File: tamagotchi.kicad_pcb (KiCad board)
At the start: 2 copper layers, 48 x 87 mm, 9 parts, among them SW1 SW_Push, SW2 SW_Push, SW3 SW_Push, U1 XIAO-ESP32-C3-SMD, U2 HS96L03W2C03

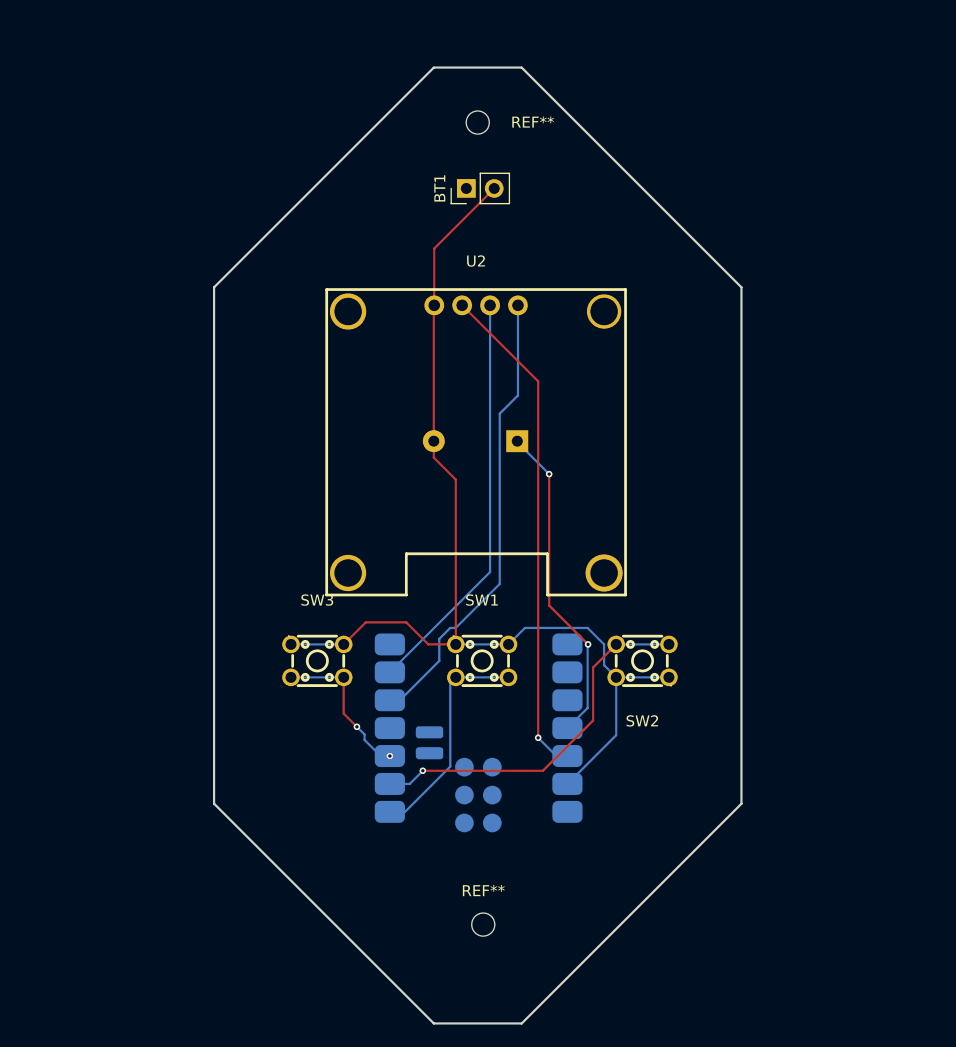
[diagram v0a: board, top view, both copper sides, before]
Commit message: Add files via upload
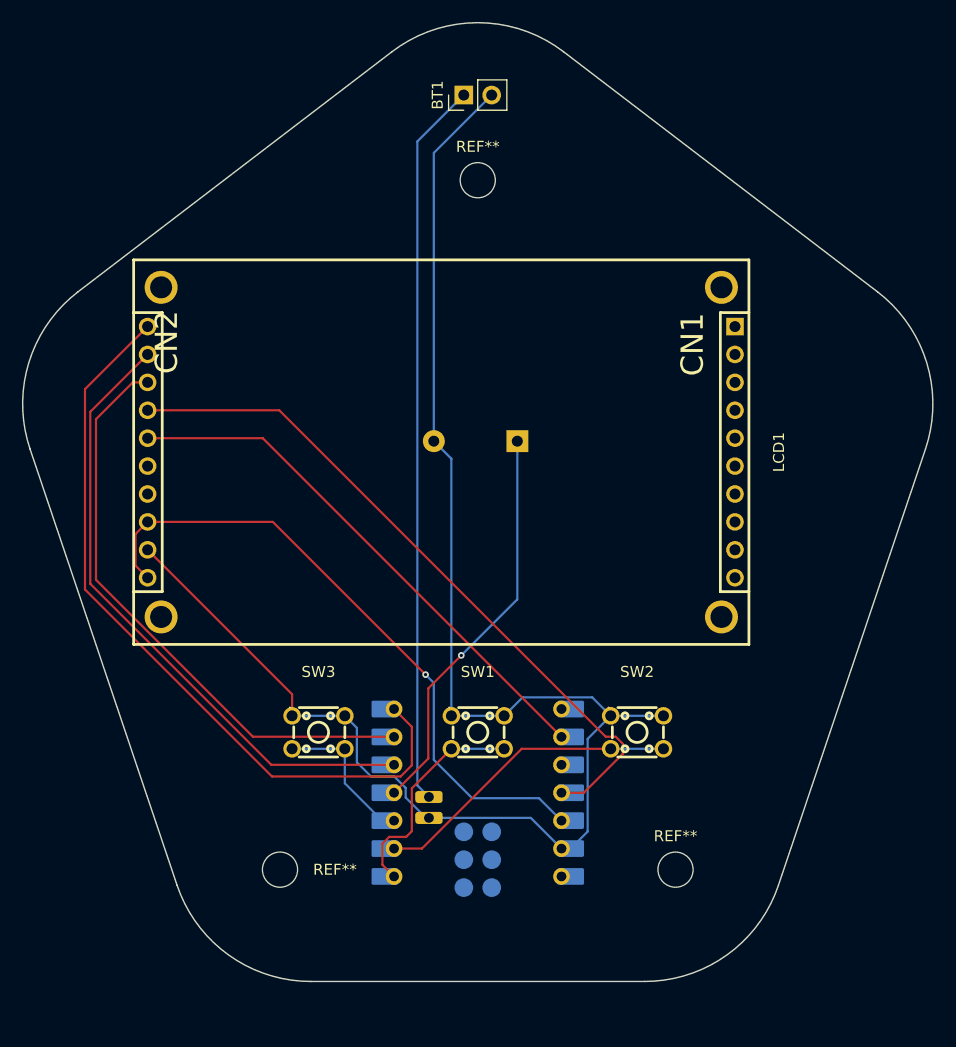
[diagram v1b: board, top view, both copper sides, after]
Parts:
- removed U2: HS96L03W2C03, easyeda2kicad:OLED-TH_L27.8-W27.2-P2.54_C9900033791
- added LCD1: HS180S10B, easyeda2kicad:LCD-TH_L56.0-W35.0-P2.54_HS180S10B, F.Cu at (127.2, 87.0)
- added REF**: MountingHole_2.1mm, MountingHole:MountingHole_2.1mm, F.Cu at (130.5, 62.2)
- U1: footprint New_XIAO_Series_Footprints:XIAO-ESP32-C3-SMD -> New_XIAO_Series_Footprints:XIAO-ESP32-C3-DIP-SMD
- moved REF** 70.3 mm to (112.5, 125.0)
- moved U1 18.6 mm to (130.5, 118.0), turned to -90 degrees
- moved REF** 18.2 mm to (148.5, 125.0)
- moved BT1 8.50 mm to (129.2, 54.5)
- moved SW2 6.52 mm to (145.0, 112.5), turned to 0 degrees
- moved SW1 6.51 mm to (130.5, 112.5)
- moved SW3 6.50 mm to (116.0, 112.5)
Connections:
- U1 pad 11: Net-(BUZZER1-+) -> Net-(U1-GPIO10_D10_MOSI)
- U1 pad 15: (no net) -> +BATT
- U1 pad 16: (no net) -> GND
- U1 pad 4: unconnected-(U1-GPIO5_A3_D3-Pad4) -> Net-(BUZZER1-+)
- U1 pad 5: Net-(U1-GPIO6_D4_SDA) -> /RES
- U1 pad 6: Net-(U1-GPIO7_D5_SCL) -> /DC
- U1 pad 7: unconnected-(U1-GPIO21_D6_TX-Pad7) -> /CS1
- U1 pad 9: unconnected-(U1-GPIO8_D8_SCK-Pad9) -> Net-(U1-GPIO8_D8_SCK)
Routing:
- net /CS1: track 0.00 -> 69.3 mm
- net +BATT: track 0.00 -> 66.1 mm
- net Net-(U1-GPIO10_D10_MOSI): track 0.00 -> 63.8 mm
- net /RES: track 0.00 -> 57.5 mm
- net /DC: track 0.00 -> 53.8 mm
- net GND: track 95.9 -> 146.9 mm
- net Net-(U1-GPIO8_D8_SCK): track 0.00 -> 48.9 mm
- net Net-(U1-GPIO6_D4_SDA): track 41.6 -> 0.00 mm
- net Net-(U1-GPIO7_D5_SCL): track 37.2 -> 0.00 mm
- net +3V3: track 45.6 -> 59.0 mm
- net Net-(BUZZER1-+): track 29.6 -> 36.6 mm, vias 2 -> 1
- net Net-(U1-GPIO3_A1_D1): track 33.5 -> 28.3 mm, vias 1 -> 0
- net Net-(U1-GPIO4_A2_D2): track 14.2 -> 13.8 mm, vias 2 -> 0
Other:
- board size 48 x 87 mm -> 82.8 x 87.3 mm
